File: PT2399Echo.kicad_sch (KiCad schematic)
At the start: 86 parts, among them Q21 2N3904, Q22 2N3904, Q23 2N3906, Q24 2N3906, SW47 SW_DPDT_x2, U28 TL074, U29 TL074, U30 LM13700, U31 PT2399

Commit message: more work...
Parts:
- C2, C3, C4, C5, C? (x8): footprint Capacitor_SMD:C_0805_2012Metric_Pad1.18x1.45mm_HandSolder -> Capacitor_SMD:C_0805_2012Metric
- C6, C7, C? (x10): footprint Capacitor_SMD:C_0805_2012Metric_Pad1.18x1.45mm_HandSolder -> Capacitor_SMD:C_0603_1608Metric
- R? (x42): footprint Resistor_SMD:R_0805_2012Metric_Pad1.20x1.40mm_HandSolder -> Resistor_SMD:R_0603_1608Metric

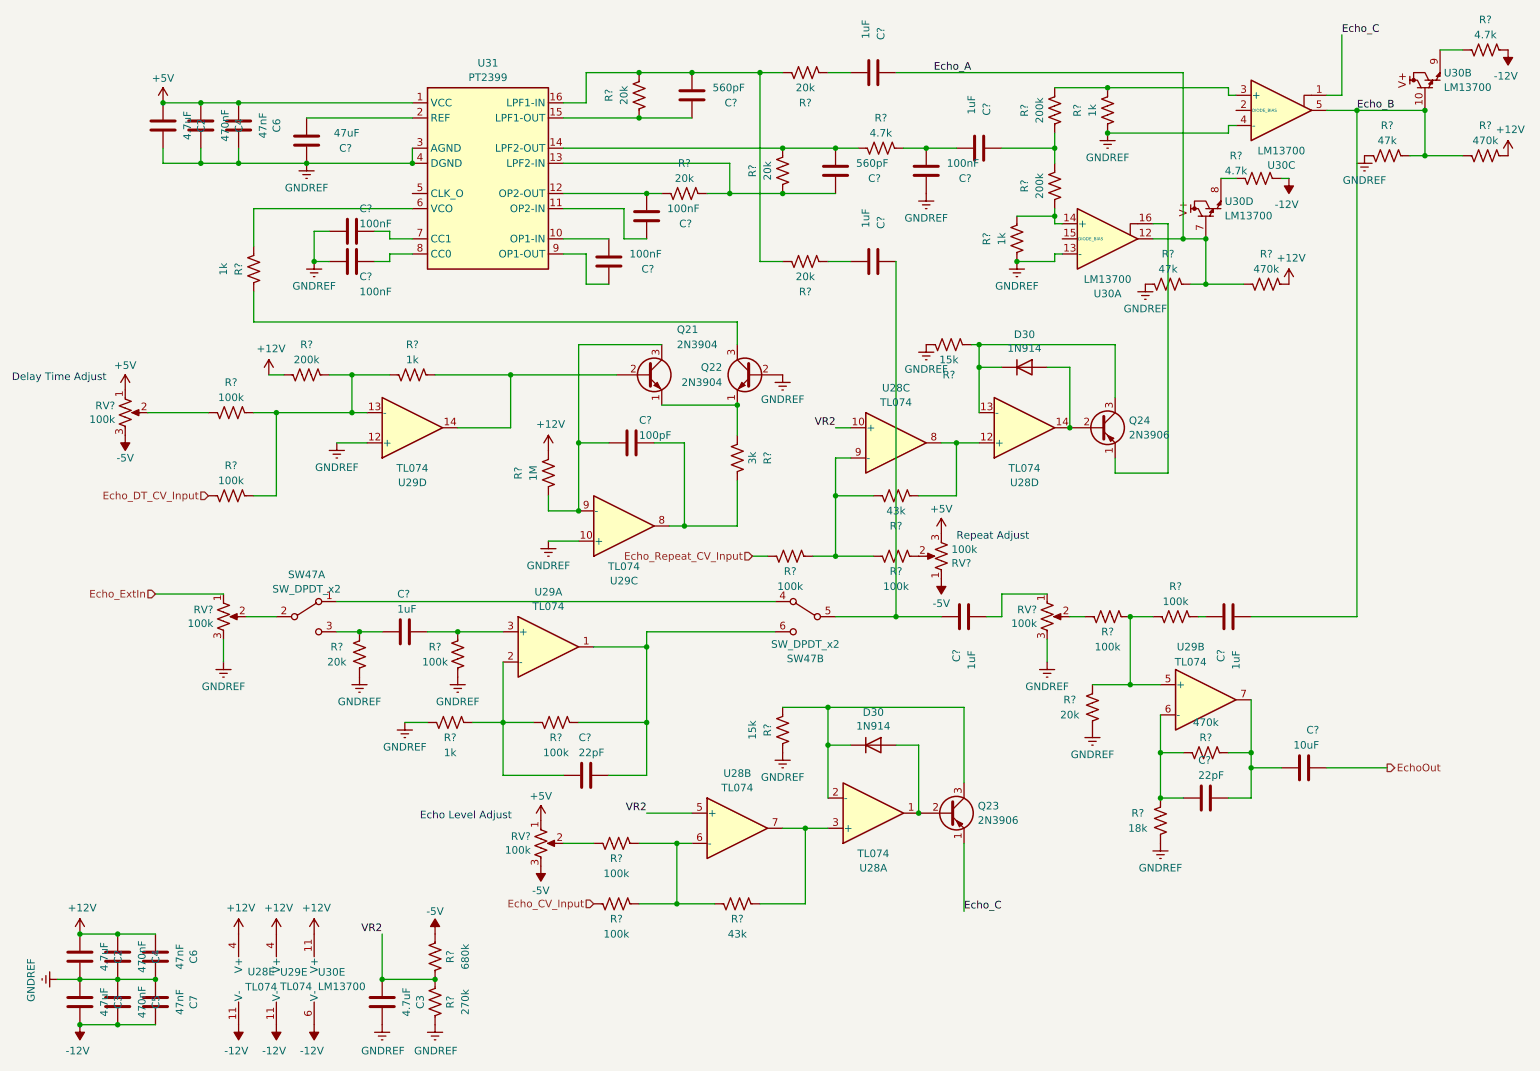
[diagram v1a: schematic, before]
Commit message: finishing schematic 1.0
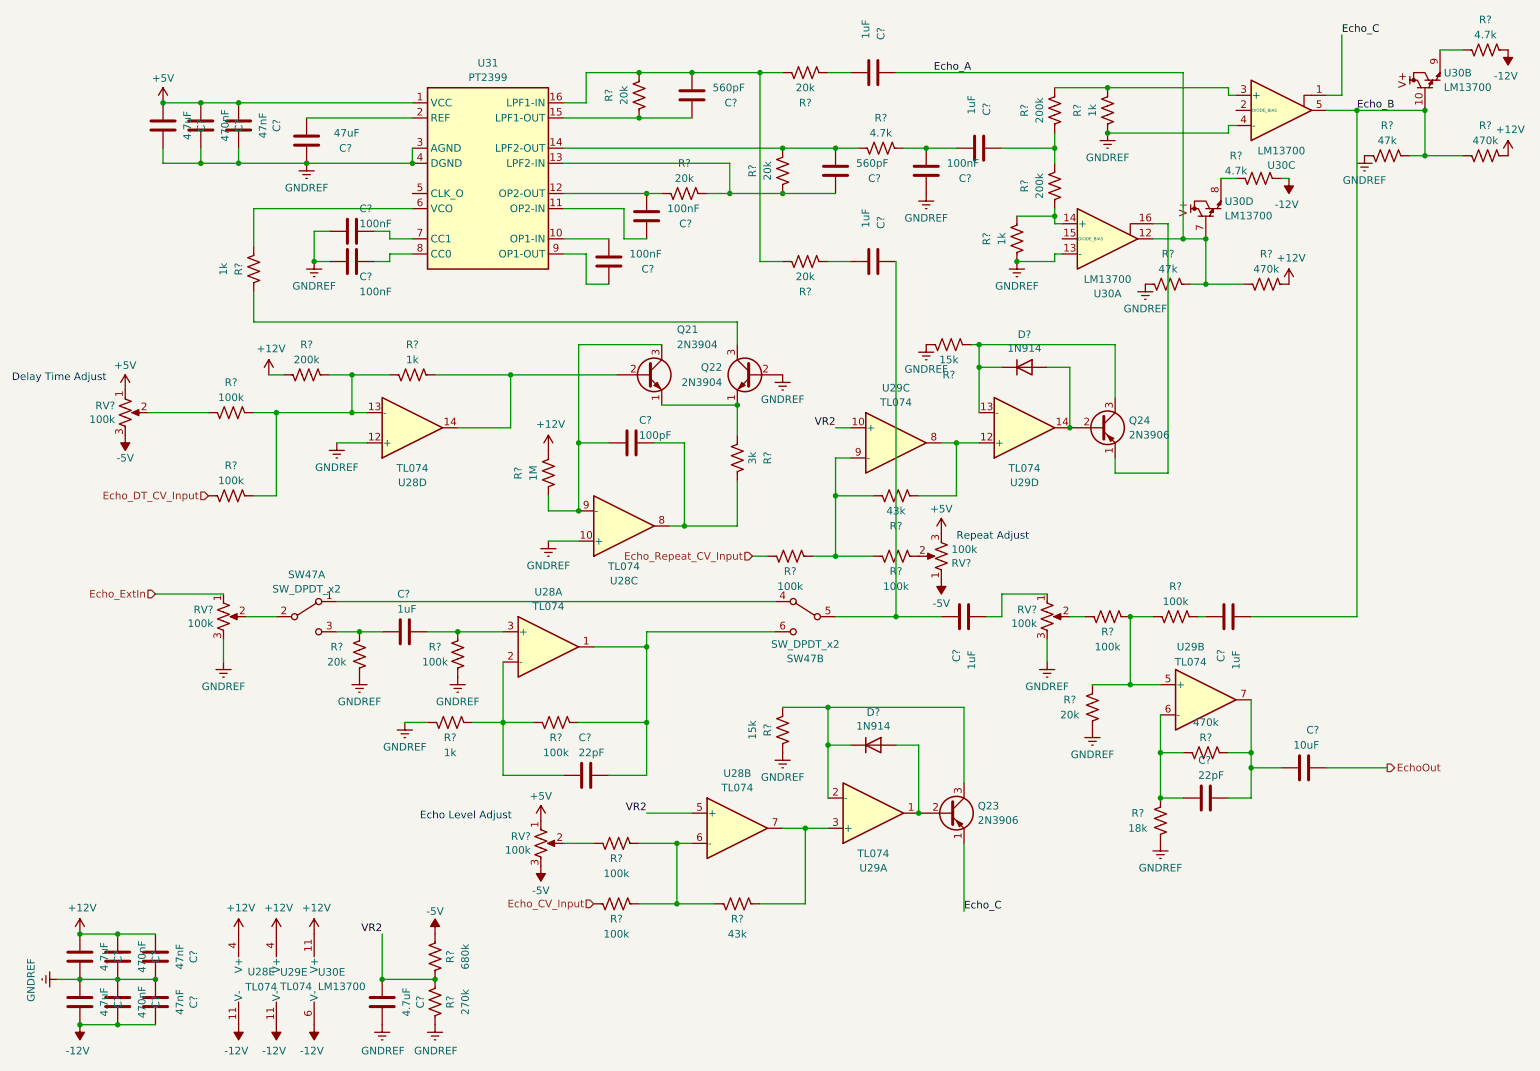
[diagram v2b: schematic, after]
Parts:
- SW47: footprint (none) -> SynthProjConnectors:MTS-203-A1-T0
- renumbered C2 to C?, C3 to C?, C7 to C?, C6 to C?, C5 to C?, C4 to C?, D30 to D?, U29 to U28, U28 to U29
